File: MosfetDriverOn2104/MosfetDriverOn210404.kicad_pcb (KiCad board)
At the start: 2 copper layers, 99.9 x 99.9 mm, 91 parts, among them J1 I2C HDR, J10 ENC, J11 CROSS CONN, J12 motor, J13 Conn_01x02_Female, J3 I2C HDR, J4 Screw_Terminal_01x02, J5 I2C HDR, J6 UART, J7 5V HDR, J8 GND, J9 servo, Q2 IRF540N, Q3 IRF540N, Q4 IRF540N, SW1 SW_Push, SW2 SW_DIP_x04, SW3 SW_Push, SW4 SW_Push, U2 L7805, U3 IR2104, U5 IR2104, U6 ATmega328P-AU-MCU_Microchip_A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

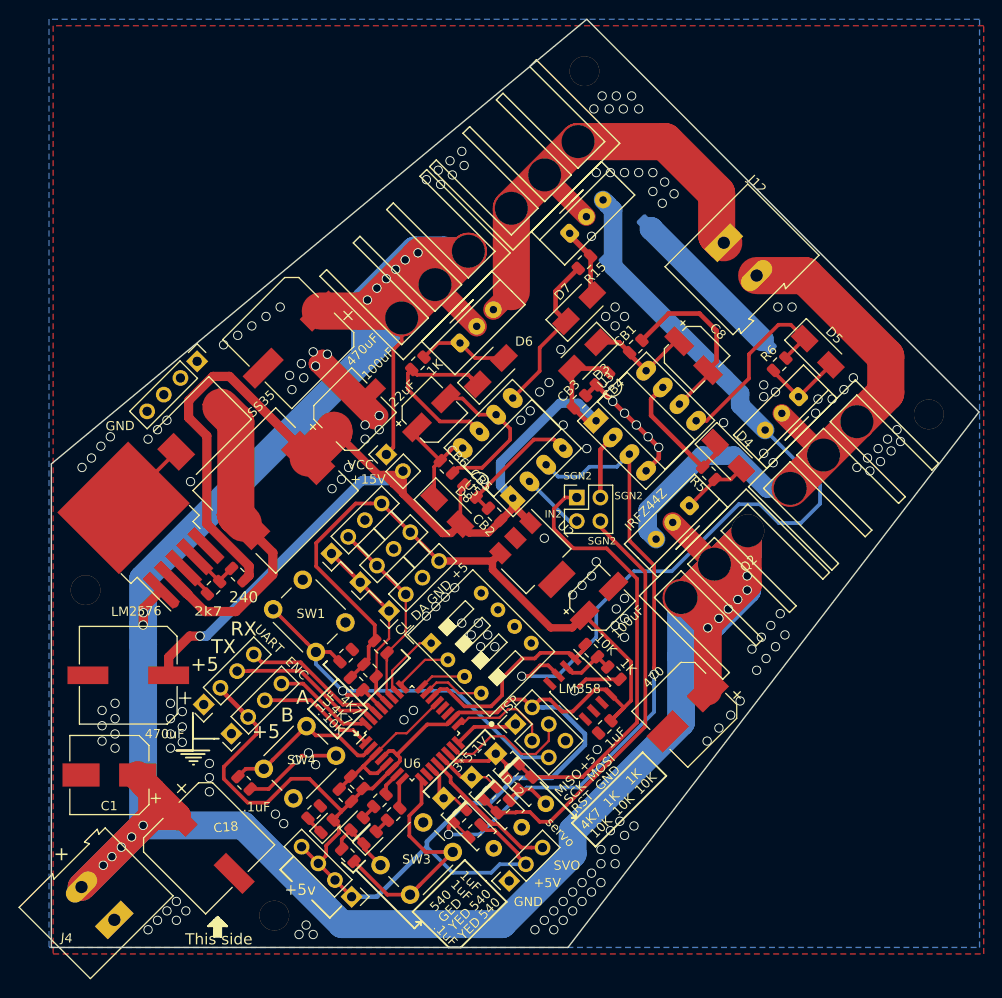
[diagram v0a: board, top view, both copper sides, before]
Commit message: #16 #15 #14 #12
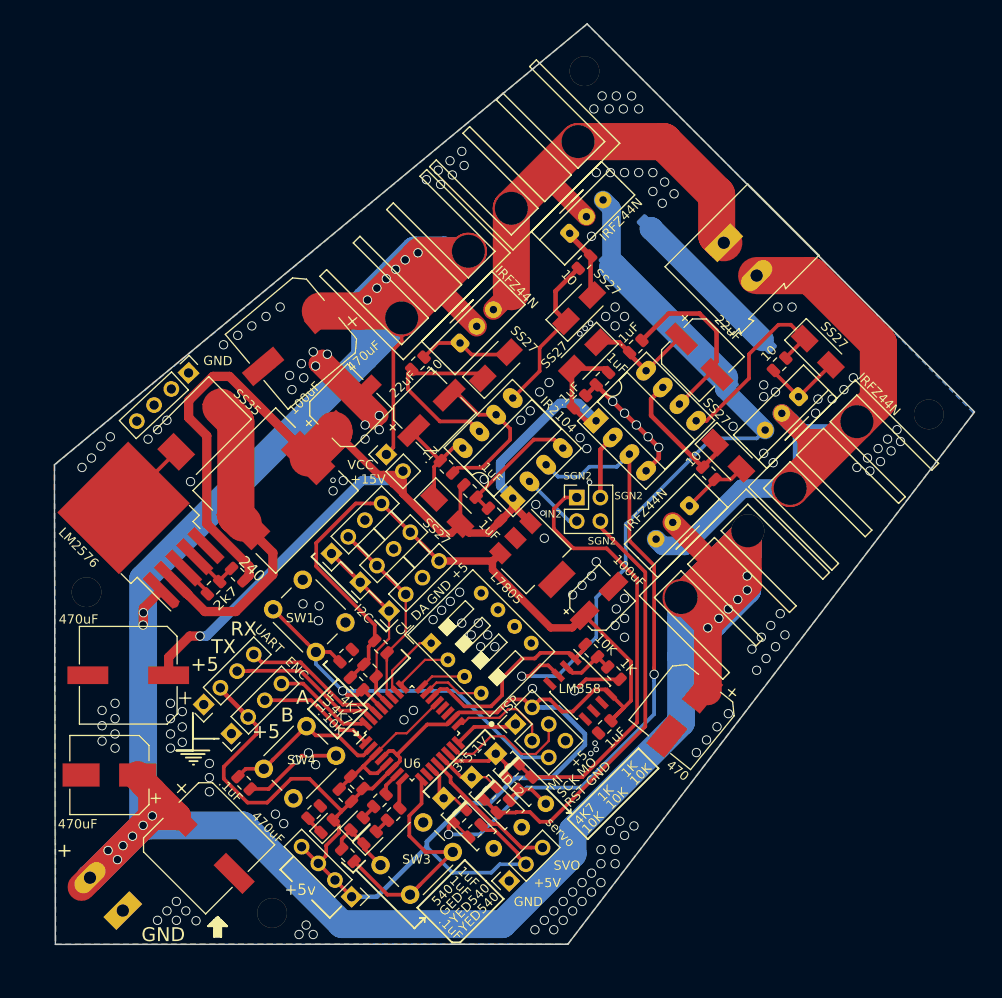
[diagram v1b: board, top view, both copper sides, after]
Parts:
- removed D6: D, Diode_SMD:D_SMA
- added SS27: D, Diode_SMD:D_SMA, F.Cu at (152.8, 88.6)
- 22uF: footprint Capacitor_SMD:CP_Elec_5x5.3 -> Capacitor_SMD:CP_Elec_6.3x5.7
- 22uF: renamed from C8; footprint Capacitor_SMD:CP_Elec_5x5.3 -> Capacitor_SMD:CP_Elec_6.3x5.7
- C1, C18: value 470 -> 470uF
- CB1: value .1 -> .1uF
- D3: value D -> SS27
- Q2, Q3, Q4: value IRF540N -> IRFZ44N
- R8: value 0E05 -> 5*0E05
- moved J8 1.55 mm to (119.7, 89.4), turned to 313 degrees
- moved J4 1.35 mm to (112.6, 147.3)
- moved 22uF 0.63 mm to (174.7, 87.7)
- moved 100uF 0.60 mm to (136.8, 93.2)
- moved C2 0.44 mm to (173.1, 126.1), turned to 231 degrees
- moved REF** 0.36 mm to (128.7, 147.6)
- moved 470uF 0.27 mm to (131.0, 85.9), turned to 220 degrees
- moved REF** 0.25 mm to (108.7, 113.0)
- renumbered R5 to 10, R6 to 10, 1K to 10, R15 to 10, IRFZ44Z to IRFZ44N, D4 to SS27, D5 to SS27, D7 to SS27
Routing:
- net /IS+: track 90.5 -> 79.3 mm
- net /M2: track 61.3 -> 51.0 mm
- net Net-(D6-Pad1): track 19.7 -> 21.1 mm
- net VCC: track 395.5 -> 394.2 mm, vias 19 -> 20
- net GND: vias 178 -> 189
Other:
- board size 99.9 x 99.9 mm -> 99.1 x 99.1 mm
- board text added: "I2C"
- board text added: "MI"
- board text added: "MO"
- board text removed: "MISO"
- board text removed: "MOSI"
- board text removed: "This side"
